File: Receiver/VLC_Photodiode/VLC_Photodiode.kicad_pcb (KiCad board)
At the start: 2 copper layers, 30 x 40 mm, 9 parts, among them J1 Screw_Terminal_01x02, J2 RF3-05-T-00-50-G, J3 RF3-05-T-00-50-G, J4 RF3-05-T-00-50-G, J5 Screw_Terminal_01x02, J6 Screw_Terminal_01x02

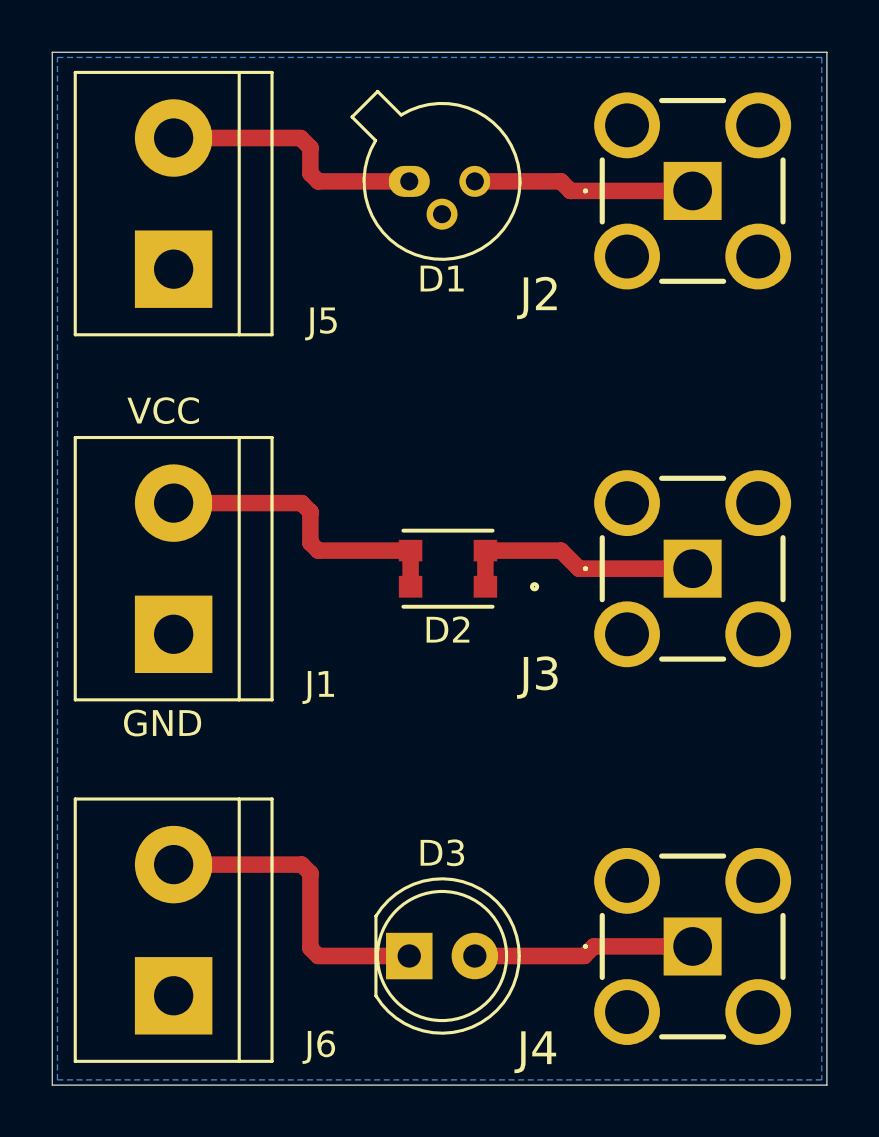
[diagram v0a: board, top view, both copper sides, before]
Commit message: Version Sma Edge
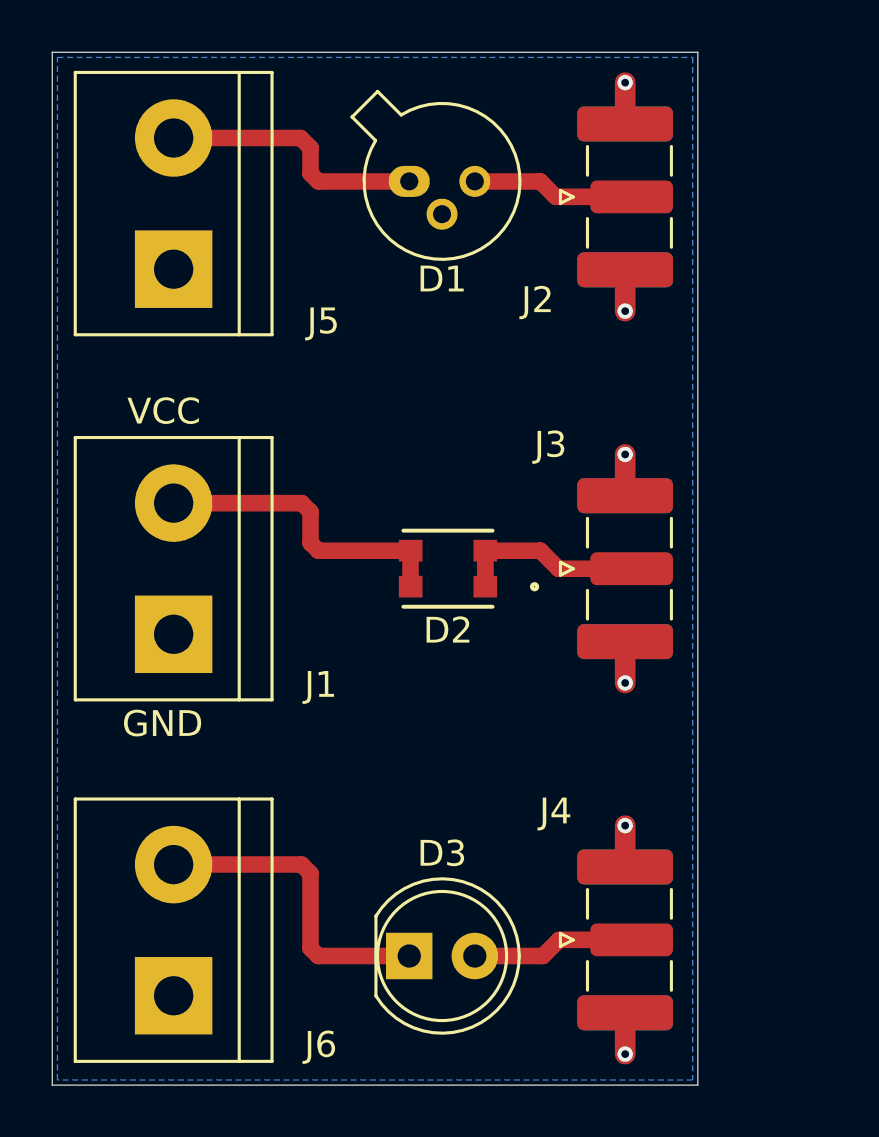
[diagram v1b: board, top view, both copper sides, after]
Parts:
- J2, J3, J4: value RF3-05-T-00-50-G -> SMA H; footprint Lumicom_Photodiode:RF305T0050G -> Connector_Coaxial:SMA_Samtec_SMA-J-P-H-ST-EM1_EdgeMount
- moved J4 2.38 mm to (122.4, 94.4)
- moved J2 2.37 mm to (122.4, 65.6)
- moved J3 2.36 mm to (122.4, 80.0)
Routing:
- net GND: track 0.00 -> 9.60 mm, vias 0 -> 6
- net Net-(J3-In): track 9.71 -> 7.35 mm
- net Net-(D1-A): track 8.59 -> 6.32 mm
- net Net-(D3-A): track 8.59 -> 6.33 mm
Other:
- board size 30 x 40 mm -> 25 x 40 mm

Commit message: v3 according to Issue #1
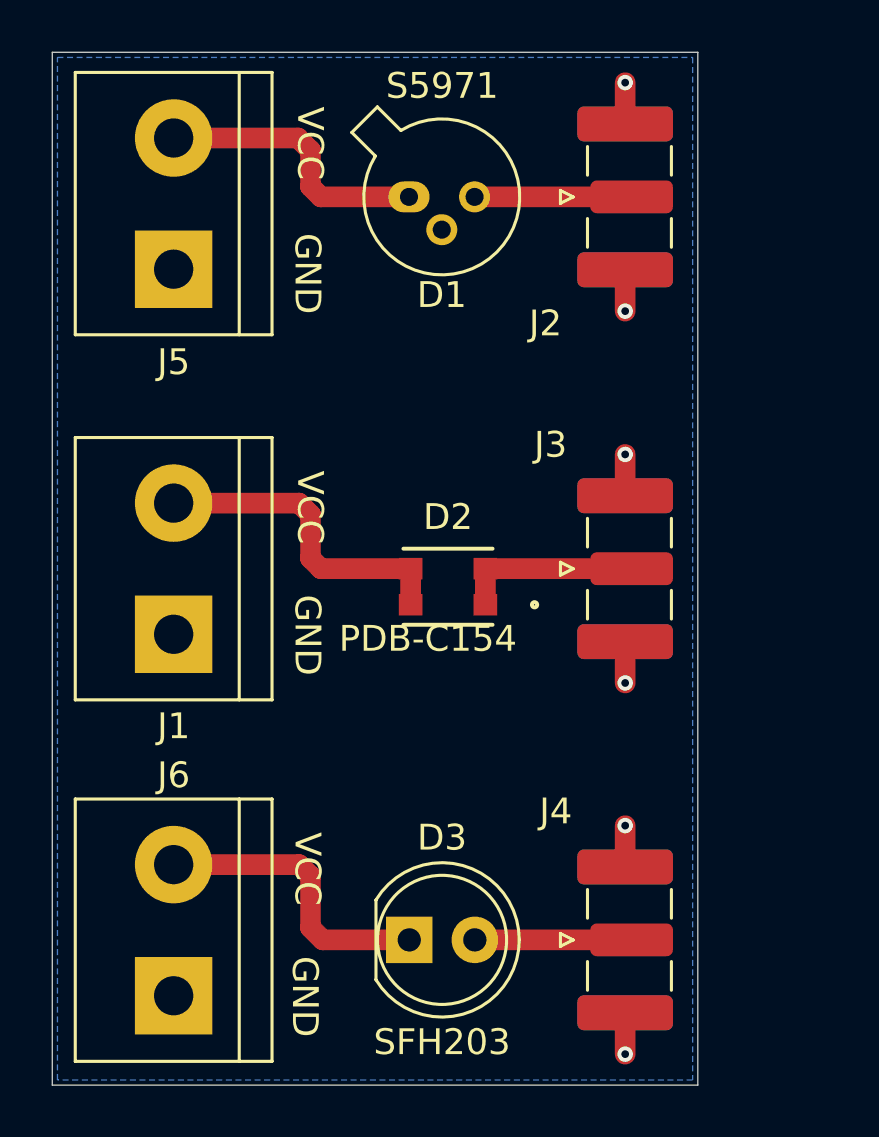
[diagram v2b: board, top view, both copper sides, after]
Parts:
- moved D2 0.70 mm to (115.3, 80.7)
- moved D3 0.62 mm to (113.8, 94.4)
- moved D1 0.60 mm to (113.8, 65.6)
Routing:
- net Net-(D3-K): track 12.3 -> 11.5 mm
- net Net-(J1-Pin_2): track 12.0 -> 12.6 mm
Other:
- board text added: "PDB-C154"
